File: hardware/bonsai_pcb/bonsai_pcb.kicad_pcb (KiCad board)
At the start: 2 copper layers, 53 x 23 mm, 6 parts, among them J1 Audio Amp Conn, J3 PH2.0 Battery Connector, SW1 BT1, U1 XIAO-ESP32-S3-SMD

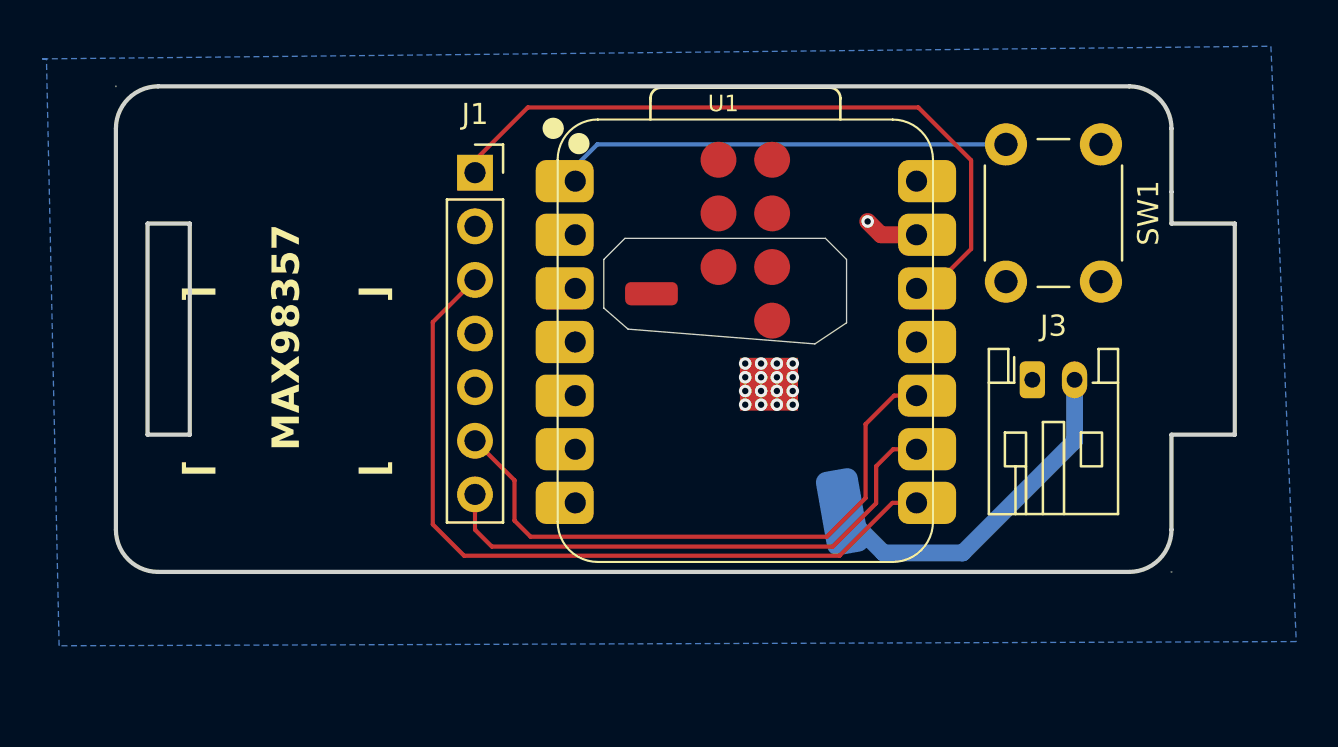
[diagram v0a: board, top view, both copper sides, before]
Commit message: Update PCB, schematic, and STEP model
Co-Authored-By: Claude Sonnet 5 <noreply@anthropic.com>
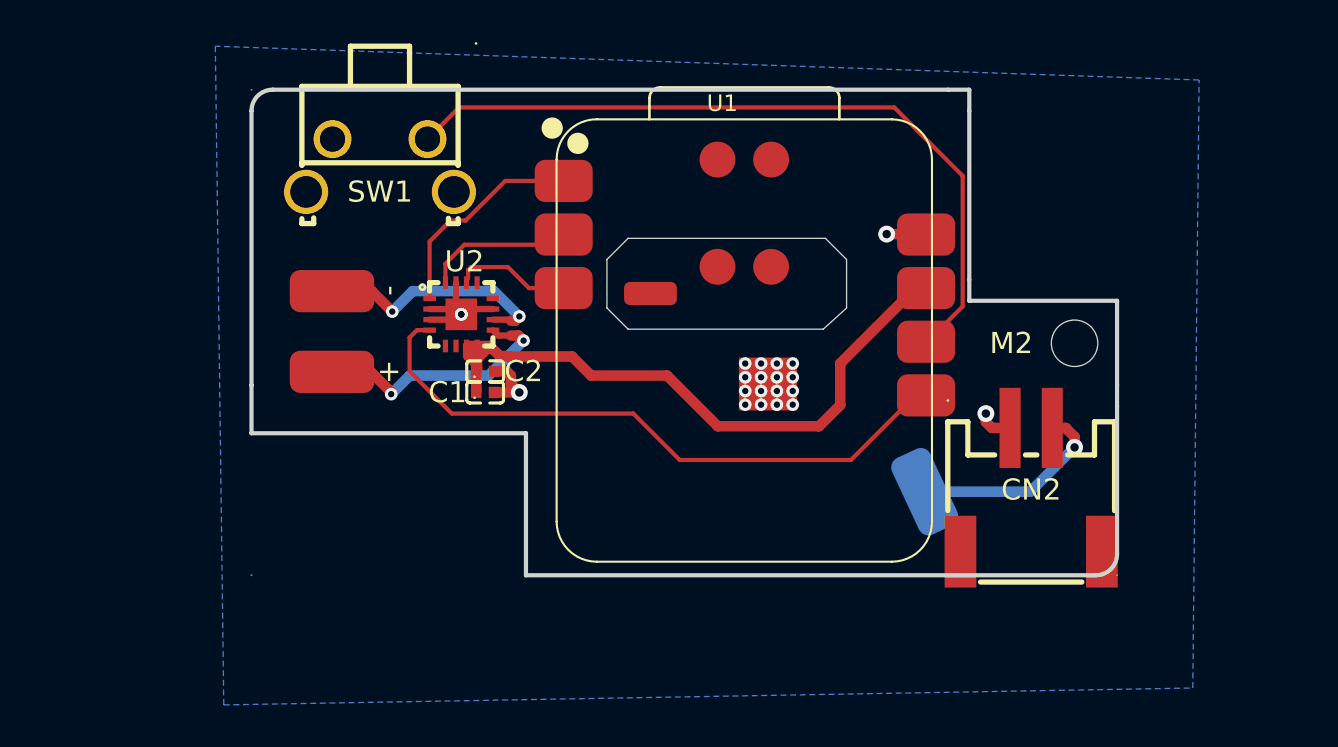
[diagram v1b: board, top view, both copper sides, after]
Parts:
- removed J1: Audio Amp Conn, Connector_PinSocket_2.54mm:PinSocket_1x07_P2.54mm_Vertical
- removed J3: PH2.0 Battery Connector, Connector_JST:JST_PH_S2B-PH-K_1x02_P2.00mm_Horizontal
- added +: Conn_01x01_Socket, Connector_Wire:SolderWirePad_1x01_SMD_2x4mm, F.Cu at (135.7, 99.0)
- added -: Conn_01x01_Socket, Connector_Wire:SolderWirePad_1x01_SMD_2x4mm, F.Cu at (135.7, 95.2)
- added C1: 10uF, JLCPCB_Capacitors:C0402, F.Cu at (143.0, 100.0)
- added C2: 100nF, JLCPCB_Capacitors:C0402, F.Cu at (143.0, 99.0)
- added CN2: S2B-PH-SM4-TB, JLCPCB_Connectors:CONN-SMD_P2.00_S2B-PH-SM4-TB-LF-SN, F.Cu at (168.8, 104.6)
- added M2: MountingHole_2.2mm_M2, MountingHole:MountingHole_2.2mm_M2, F.Cu at (170.9, 97.7)
- added U2: MAX98357AETE+T, JLCPCB_Amplifiers:TQFN-16_L3.0-W3.0-P0.50-BL-EP1.5, F.Cu at (141.8, 96.3)
- SW1: value BT1 -> TS-1102N-5516; footprint Button_Switch_THT:SW_PUSH_6mm -> JLCPCB_Switches:SW-TH_TS-1102N-5516
- moved SW1 30.2 mm to (138.0, 89.2), turned to 180 degrees
- moved J2 4.01 mm to (163.8, 104.7), turned to -155 degrees
- moved G*** 3.60 mm to (138.6, 94.1)
- renumbered B+ to J2
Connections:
- U1 pad 1: BT1 -> DIN
- U1 pad 10: BLCK -> SD
- U1 pad 2: unconnected-(U1-GPIO2_A1_D1-Pad2) -> BLCK
- U1 pad 3: unconnected-(U1-GPIO3_A2_D2-Pad3) -> LRC
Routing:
- net BLCK: track 28.7 -> 7.57 mm
- net LRC: track 25.8 -> 5.90 mm
- net BT1: track 21.5 -> 36.4 mm
- net /OUTP: track 0.00 -> 12.3 mm, vias 0 -> 2
- net /OUTN: track 0.00 -> 11.5 mm, vias 0 -> 2
- net DIN: track 0.00 -> 10.7 mm
- net GND: track 2.58 -> 12.1 mm, vias 17 -> 21
- net SD: track 37.0 -> 29.7 mm
- net Net-(J2-Pin_1): track 16.9 -> 9.70 mm, vias 0 -> 1
- net VIN: track 33.0 -> 31.1 mm
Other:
- board size 53 x 23 mm -> 41 x 23 mm
- board text removed: "⌈ ⌉ MAX98357 ⌊ ⌋"
